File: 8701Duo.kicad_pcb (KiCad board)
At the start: 2 copper layers, 19.5 x 21 mm, 12 parts, among them J1 Clock, U1 ICS525-01R, U2 MOS8701, U3 74LVC1G06, X1 LFSPXO021772Bulk, X2 LFSPXO020648Bulk

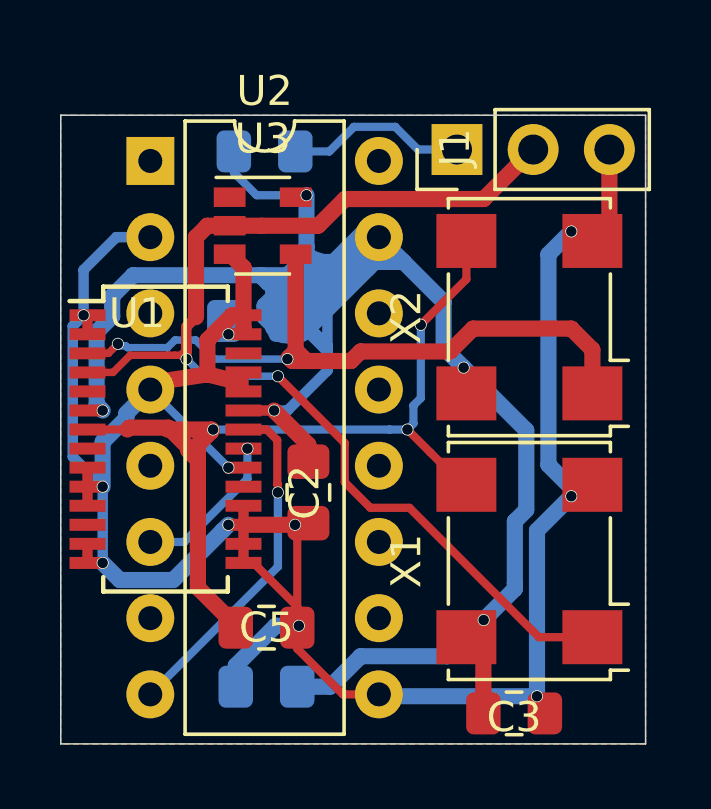
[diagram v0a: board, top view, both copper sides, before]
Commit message: Add files via upload
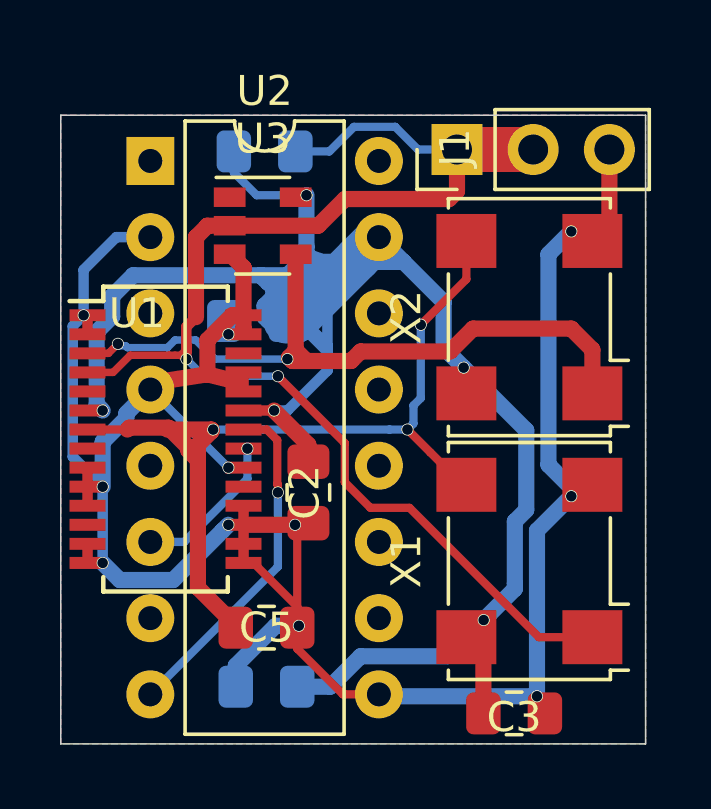
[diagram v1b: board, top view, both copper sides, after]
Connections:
- J1 pad 2: Net-(J1-Pad2) -> Net-(J1-Pad1)
- U1 pad 4: Net-(J1-Pad2) -> Net-(J1-Pad1)
- U3 pad 2: Net-(J1-Pad2) -> Net-(J1-Pad1)
- X1 pad 1: Net-(J1-Pad2) -> Net-(J1-Pad1)
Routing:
- net Net-(J1-Pad1): track 6.04 -> 46.3 mm, vias 0 -> 2
- net Net-(J1-Pad2): track 39.4 -> 0.00 mm, vias 2 -> 0
